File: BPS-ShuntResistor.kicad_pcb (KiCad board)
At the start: 2 copper layers, 40.1 x 35.1 mm, 15 parts, among them J3 Amp_Conn

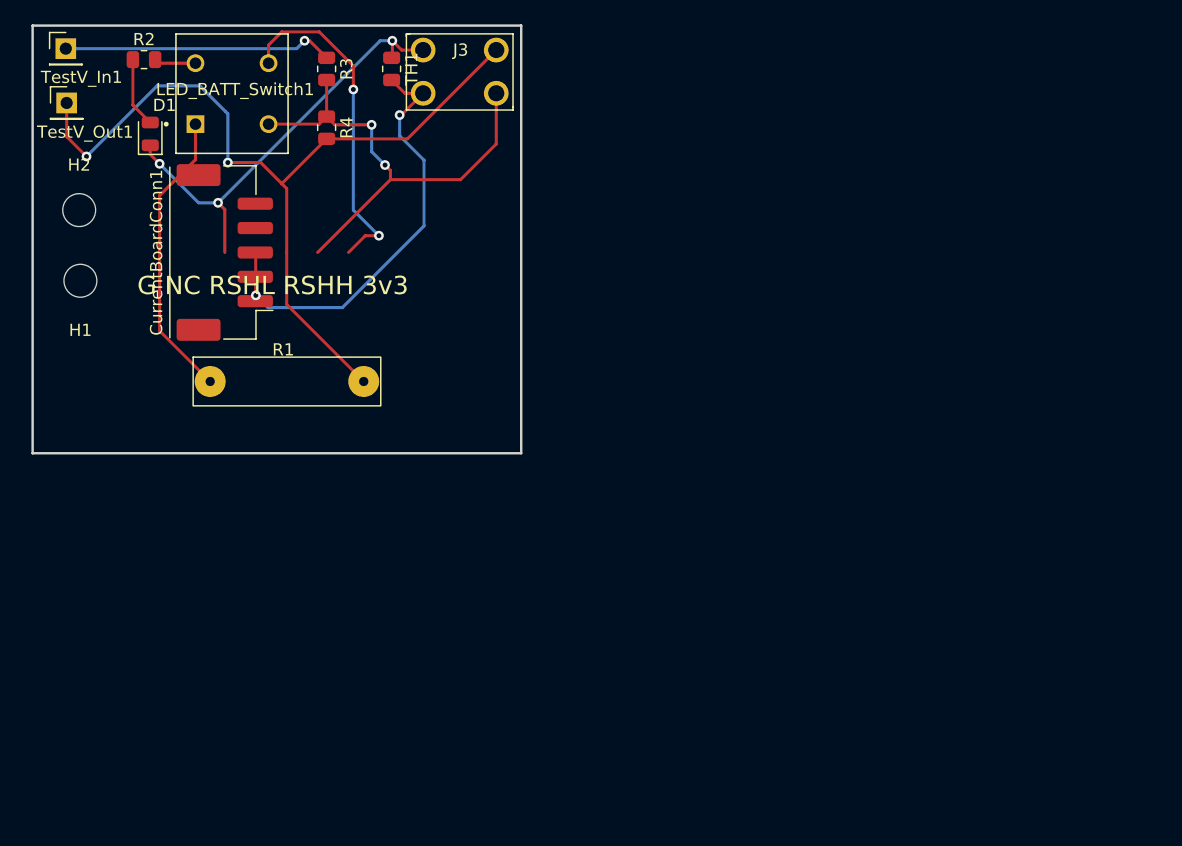
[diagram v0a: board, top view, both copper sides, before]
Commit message: Working on new layout
Kind of messy
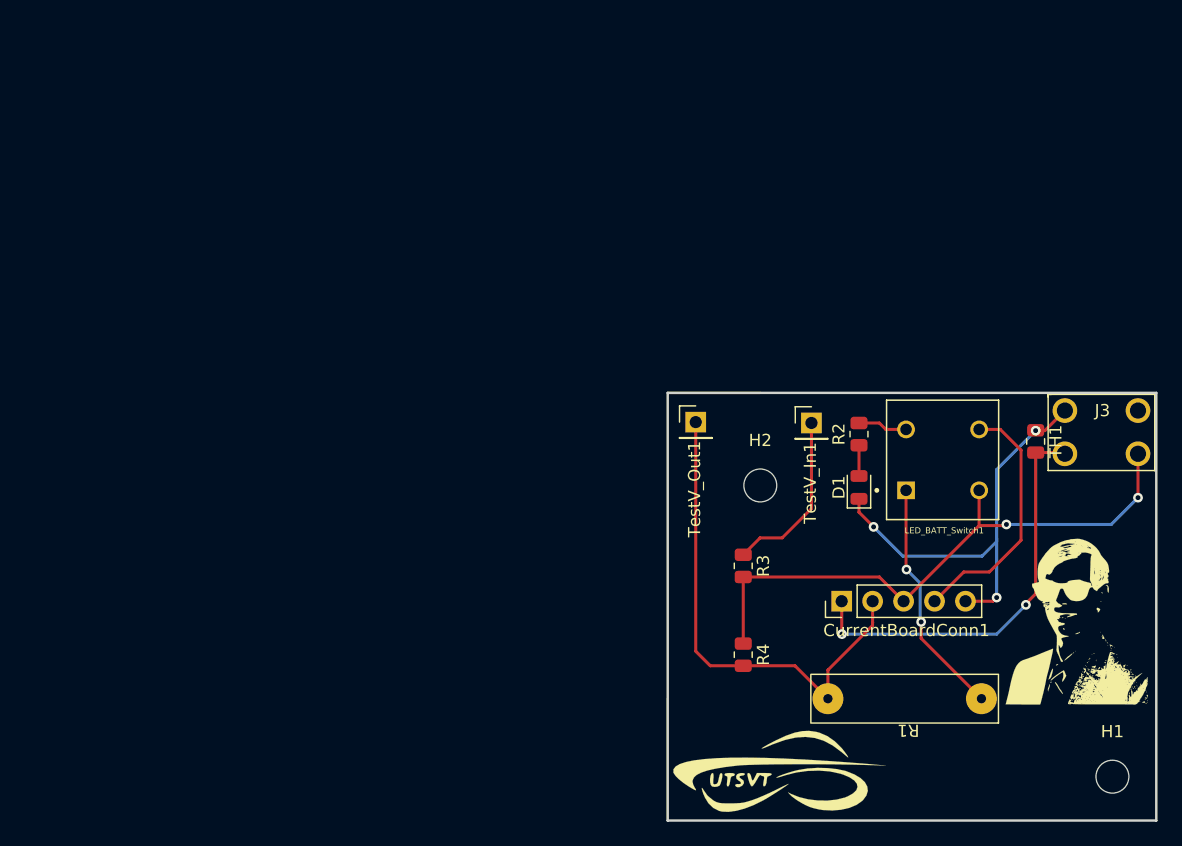
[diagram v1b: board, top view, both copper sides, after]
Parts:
- CurrentBoardConn1: footprint Connector_Molex:Molex_CLIK-Mate_502443-0570_1x05-1MP_P2.00mm_Vertical -> Connector_PinHeader_2.54mm:PinHeader_1x05_P2.54mm_Vertical
- LOGO1, LOGO2: moved to F.Cu
- moved H1 94.0 mm to (153.9, 116.0)
- moved TestV_In1 68.5 mm to (129.2, 87.0)
- moved R2 66.2 mm to (133.1, 87.9), turned to 90 degrees
- moved LED_BATT_Switch1 65.6 mm to (140.0, 90.0)
- moved D1 65.0 mm to (133.1, 92.3)
- moved TH1 61.1 mm to (147.6, 88.5)
- moved J3 60.4 mm to (153.0, 87.5)
- moved H2 60.3 mm to (125.0, 92.1)
- moved CurrentBoardConn1 58.2 mm to (131.7, 101.6)
- moved TestV_Out1 57.9 mm to (119.7, 86.9)
- moved R1 57.5 mm to (137.2, 109.6), turned to 180 degrees
- moved LOGO2 56.4 mm to (150.5, 103.1), turned to 0 degrees
- moved R4 55.1 mm to (123.6, 106.0)
- moved LOGO1 54.9 mm to (126.3, 115.7), turned to 0 degrees
- moved R3 53.2 mm to (123.6, 98.7)
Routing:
- net RSHL: track 70.3 -> 40.8 mm, vias 2 -> 0
- net RSHH: track 39.6 -> 48.7 mm
- net Net-(R3-Pad1): track 22.3 -> 14.2 mm, vias 1 -> 0
- net +3V3: track 27.9 -> 20.7 mm, vias 2 -> 0
- net Net-(LED_BATT_Switch1-Pad1): track 24.1 -> 19.7 mm, vias 0 -> 2
- net Net-(D1-Pad2): track 5.75 -> 2.53 mm
- net ETS: track 36.2 -> 34.1 mm
- net GND: track 36.3 -> 35.4 mm
- net Net-(LED_BATT_Switch1-Pad3): track 3.43 -> 4.08 mm
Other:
- board text removed: "G NC RSHL RSHH 3v3"
